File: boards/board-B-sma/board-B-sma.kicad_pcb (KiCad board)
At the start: 4 copper layers, 74.8 x 149.1 mm, 30 parts, among them J5 SAMTEC_QSE-040-01-X-D-A, K0 SMA_Amphenol_901-143_Horizont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, K1 SMA_Amphenol_901-143_Horizont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, K10 SMA_Amphenol_901-143_Horizont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, K11 SMA_Amphenol_901-143_Horizont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, K12 SMA_Amphenol_901-143_Horizont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, K13 SMA_Amphenol_901-143_Horizont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, K14 SMA_Amphenol_901-143_Horizont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, K15 SMA_Amphenol_901-143_Horizont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, K16 SMA_Amphenol_901-143_Horizont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, K17 SMA_Amphenol_901-143_Horizont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, K18 SMA_Amphenol_901-143_Horizont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, K19 SMA_Amphenol_901-143_Horizont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, K2 SMA_Amphenol_901-143_Horizont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, K20 SMA_Amphenol_901-143_Horizont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, K21 SMA_Amphenol_901-143_Horizont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, K22 SMA_Amphenol_901-143_Horizont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, K23 SMA_Amphenol_901-143_Horizont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, K3 SMA_Amphenol_901-143_Horizont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, K4 SMA_Amphenol_901-143_Horizont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, K5 SMA_Amphenol_901-143_Horizont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, K6 SMA_Amphenol_901-143_Horizont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, K7 SMA_Amphenol_901-143_Horizont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, K8 SMA_Amphenol_901-143_Horizont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, K9 SMA_Amphenol_901-143_Horizont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

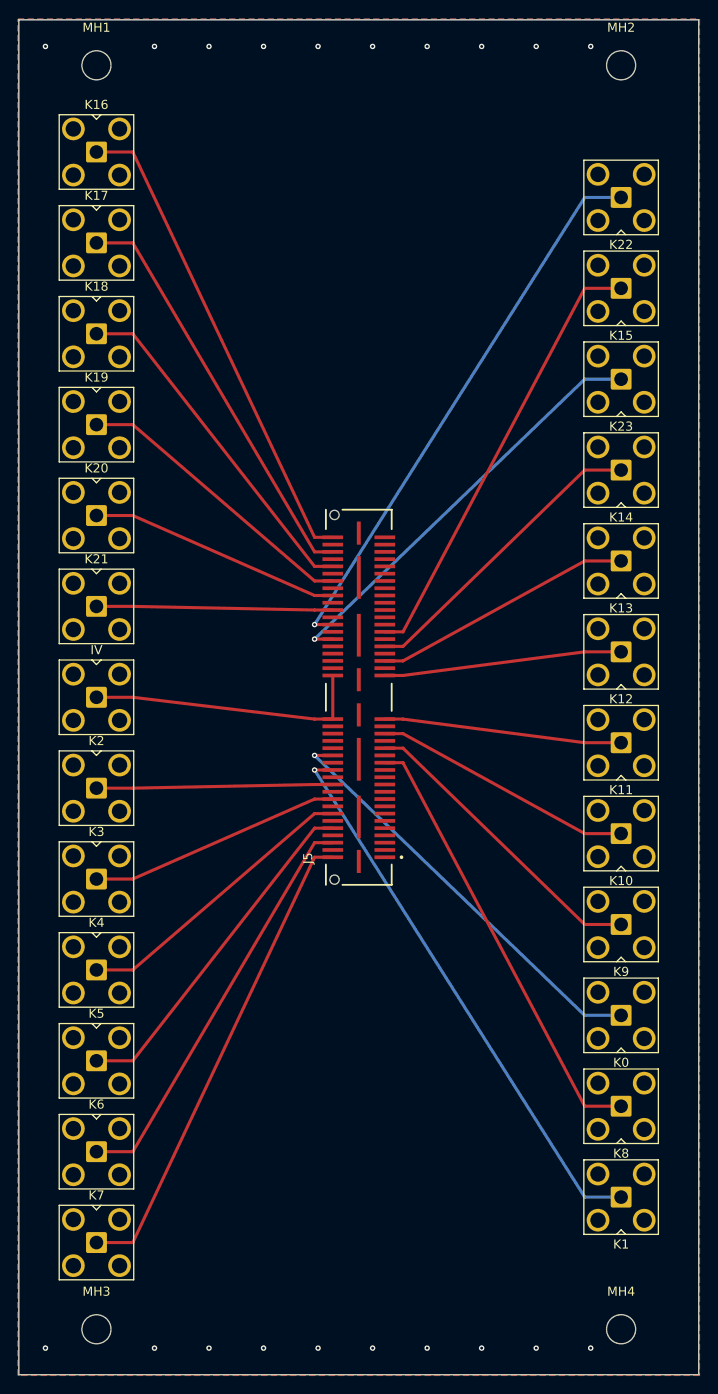
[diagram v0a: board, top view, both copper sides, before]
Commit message: initial upload
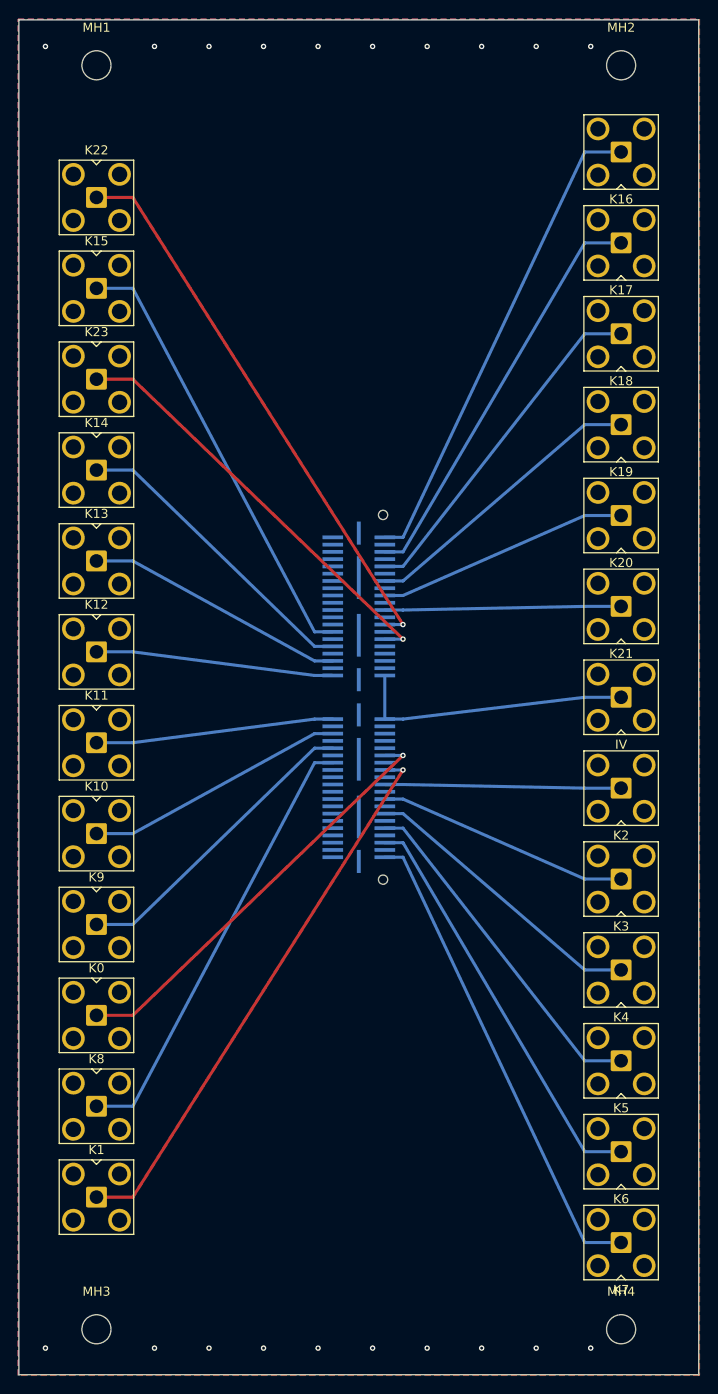
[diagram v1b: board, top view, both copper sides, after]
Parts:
- J5: moved to B.Cu
- moved IV 57.7 mm to (75.3, 84.5), turned to 90 degrees
- moved K0 57.7 mm to (17.5, 119.5), turned to -90 degrees
- moved K1 57.7 mm to (17.5, 139.5), turned to -90 degrees
- moved K10 57.7 mm to (17.5, 99.5), turned to -90 degrees
- moved K11 57.7 mm to (17.5, 89.5), turned to -90 degrees
- moved K12 57.7 mm to (17.5, 79.5), turned to -90 degrees
- moved K13 57.7 mm to (17.5, 69.5), turned to -90 degrees
- moved K14 57.7 mm to (17.5, 59.5), turned to -90 degrees
- moved K15 57.7 mm to (17.5, 39.5), turned to -90 degrees
- moved K16 57.7 mm to (75.3, 24.5), turned to 90 degrees
- moved K17 57.7 mm to (75.3, 34.5), turned to 90 degrees
- moved K18 57.7 mm to (75.3, 44.5), turned to 90 degrees
- moved K19 57.7 mm to (75.3, 54.5), turned to 90 degrees
- moved K2 57.7 mm to (75.3, 94.5), turned to 90 degrees
- moved K20 57.7 mm to (75.3, 64.5), turned to 90 degrees
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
